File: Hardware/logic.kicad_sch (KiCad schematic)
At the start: 78 parts, among them J301 Ref Divider, J302 GPS ANT, J303 Encoder, J304 Ref Select, J305 Ref Range, J306 GPS Module, J307 LCD, J308 RF 50 Ohm, J309 RF TTL, J310 1PPS TTL, J311 ICSP, J312 Serial, J313 Program, Q301 2N3904, U301 DAC8571IDGK, U302 NEO-M8M, U303 OP07, U304 OP07, U305 TXS0108EPW, U306 GALI-52, U307 74LVC1G17, U308 74LVC1G17, U309 MCP23017_SO, U310 MAX232, U311 PIC18F27Q43, U312 24AA04

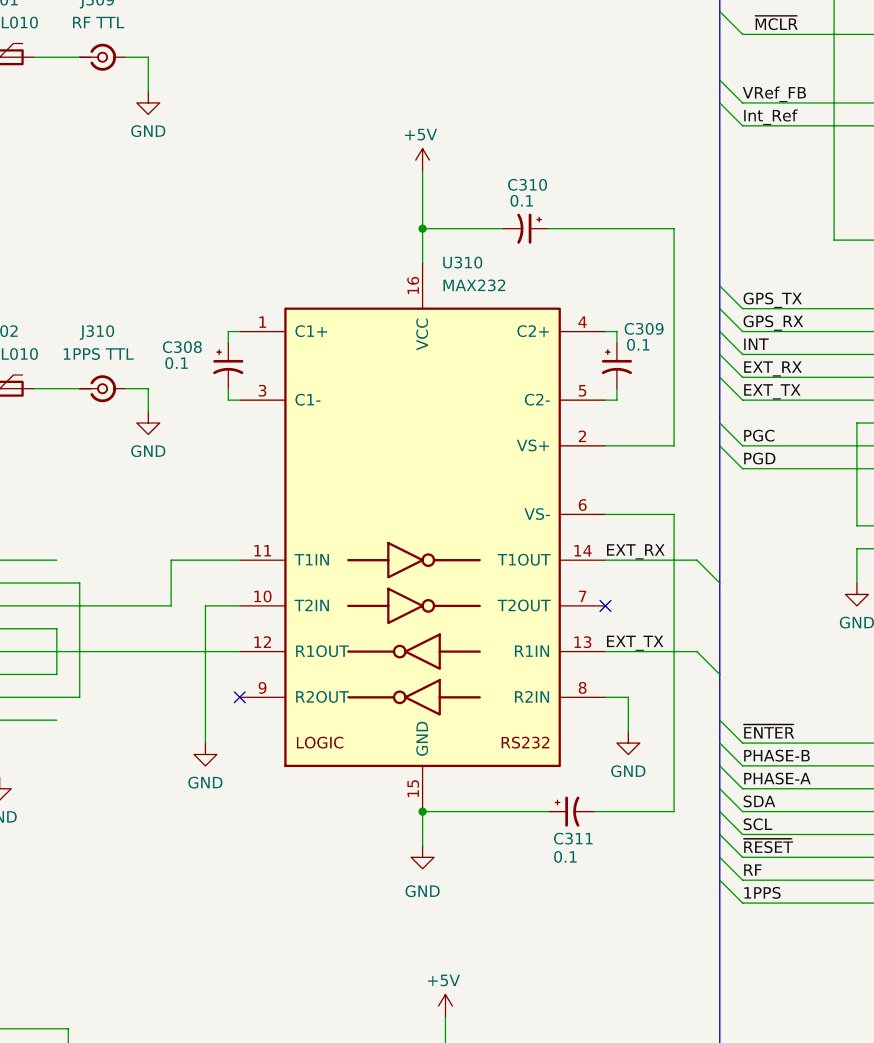
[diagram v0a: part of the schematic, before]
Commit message: LCD now working
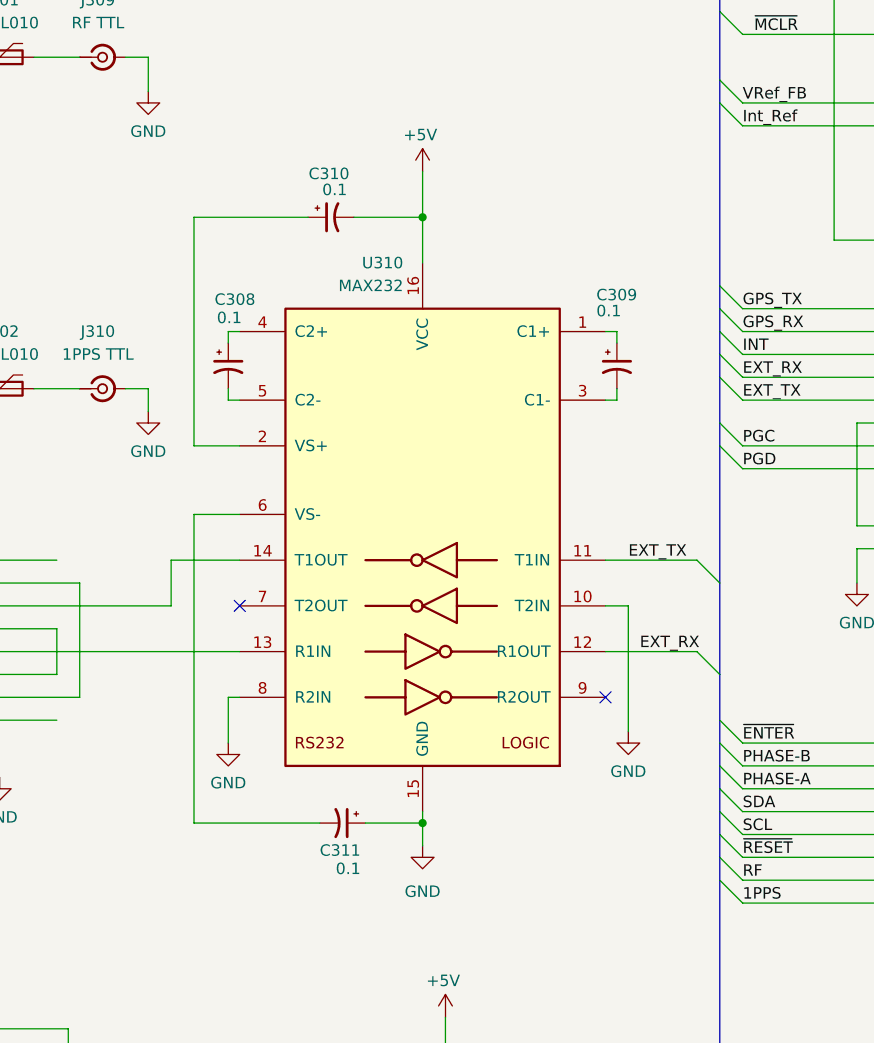
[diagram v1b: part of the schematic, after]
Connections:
- net EXT_RX: now also U310.12 (R1OUT); no longer U310.14 (T1OUT)
- net EXT_TX: now also U310.11 (T1IN); no longer U310.13 (R1IN)
- net RXD: now also U310.14 (T1OUT); no longer U310.11 (T1IN)
- net TXD: now also U310.13 (R1IN); no longer U310.12 (R1OUT)
- net at U310.1 (C1+): now also C309.1; no longer C308.1
- net at U310.3 (C1-): now also C309.2; no longer C308.2
- net at U310.4 (C2+): now also C308.1; no longer C309.1
- net at U310.5 (C2-): now also C308.2; no longer C309.2
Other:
- moved on the sheet: C310, C311
